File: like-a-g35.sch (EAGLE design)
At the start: 17 parts, among them J1 AVR_SPI_PRG_62X3_LOCK, Q1 16MHz, X1 S1, X2 S2, X3 S3, X4 POWER

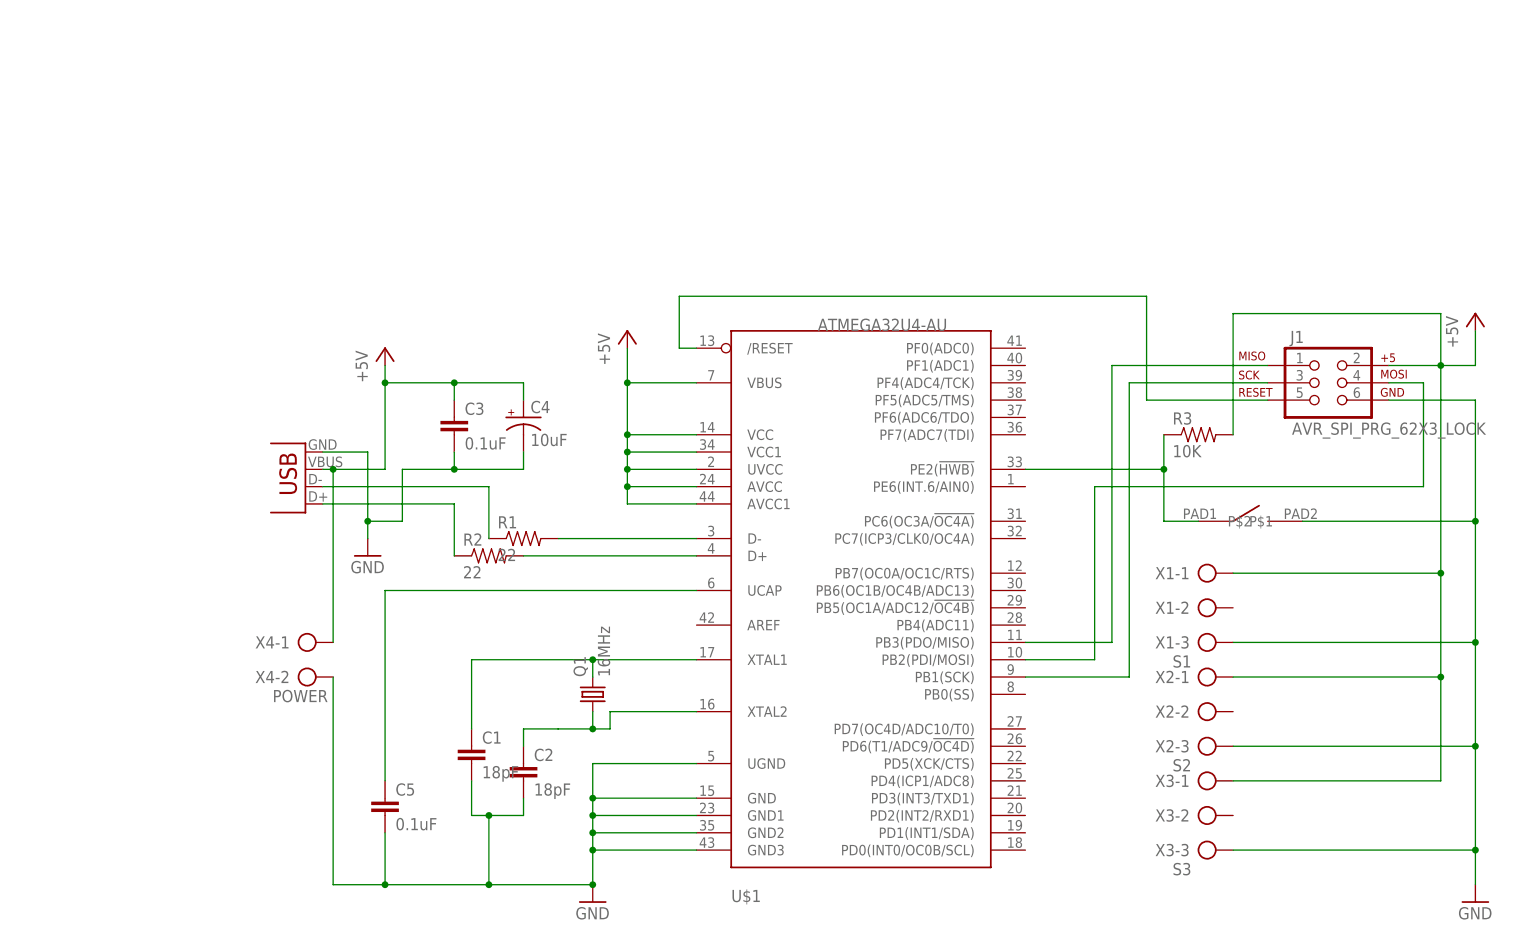
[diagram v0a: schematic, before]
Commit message: 0.9.
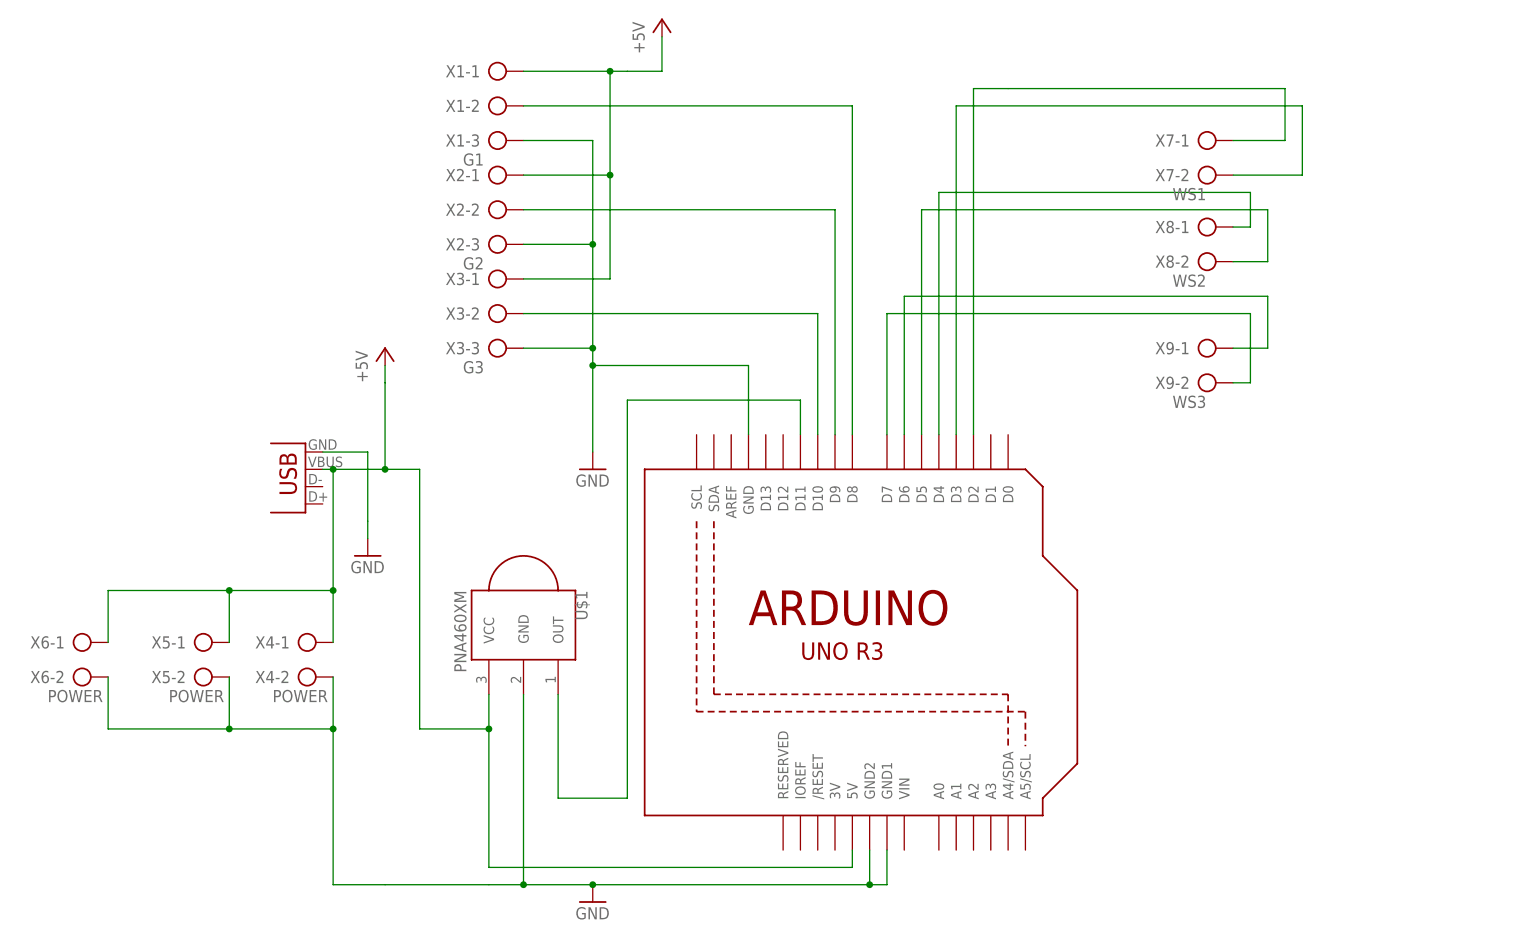
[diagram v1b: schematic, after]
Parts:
- removed C1, C2: 18pF, programmer:CAP0805
- removed C3, C5: 0.1uF, programmer:CAP0805
- removed C4: 10uF, programmer:CAP_POL1206
- removed J1: AVR_SPI_PRG_62X3_LOCK, programmer:AVR_SPI_PRG_62X3_LOCK
- removed Q1: 16MHz, crystal:CRYSTALHC49S
- removed R1, R2: 22, like-a-g35:RESISTOR0805-RES
- removed R3: 10K, like-a-g35:RESISTOR0805-RES
- removed U$3: BUTTON_TD-85XU, programmer:BUTTON_TD-85XU
- added U1: ARDUINOR3-DIMENSION, adafruit:ARDUINOR3-DIMENSION
- added X5, X6: POWER, con-ptr500:AK300/2
- added X7: WS1, con-ptr500:AK300/2
- added X8: WS2, con-ptr500:AK300/2
- added X9: WS3, con-ptr500:AK300/2
- U$1: value ATMEGA32U4-AU -> PNA460XM; device like-a-g35:ATMEGA32U4-AU -> adafruit:PNA460XM
- X1: value S1 -> G1
- X2: value S2 -> G2
- X3: value S3 -> G3
- renumbered U$2 to U2
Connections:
- removed net !RESET: J1.5, U$1./RESET
- removed net 3V3: C5.1, U$1.UCAP
- removed net D+: R2.2, U$1.D+
- removed net D-: R1.2, U$1.D-
- removed net MISO: J1.1, U$1.PB3(PDO/MISO)
- removed net MOSI: J1.4, U$1.PB2(PDI/MOSI)
- removed net N$1: R3.1, U$1.PE2(!HWB), U$3.P$1
- removed net RAW_D+: R2.1, U2.D+
- removed net RAW_D-: R1.1, U2.D-
- removed net SCK: J1.3, U$1.PB1(SCK)
- removed net XTAL1: C1.1, Q1.2, U$1.XTAL1
- removed net XTAL2: C2.1, Q1.1, U$1.XTAL2
- new net CLK1: U1.D3, X7-2.KL
- new net CLK2: U1.D5, X8-2.KL
- new net CLK3: U1.D7, X9-2.KL
- new net DATA1: U1.D2, X7-1.KL
- new net DATA2: U1.D4, X8-1.KL
- new net DATA3: U1.D6, X9-1.KL
- new net GDATA1: U1.D8, X1-2.KL
- new net GDATA2: U1.D9, X2-2.KL
- new net GDATA3: U1.D10, X3-2.KL
- new net IR-OUT: U$1.OUT, U1.D11
- net +5V: now also U1.5V, X5-1.KL, X6-1.KL; no longer C3.1, C4.+, J1.2, R3.2, U$1.AVCC, U$1.AVCC1, U$1.UVCC, U$1.VBUS, U$1.VCC1
- net GND: now also U1.GND, U1.GND1, U1.GND2, X5-2.KL, X6-2.KL; no longer C1.2, C2.2, C3.2, C4.-, C5.2, J1.6, U$1.GND1, U$1.GND2, U$1.GND3, U$1.UGND, U$3.P$2
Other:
- moved on the sheet: X1-1, X1-2, X1-3, X2-1, X2-2, X2-3, X3-1, X3-2, X3-3
